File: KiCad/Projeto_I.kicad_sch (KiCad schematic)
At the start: 43 parts, among them J1 PORTA, J2 PORTB, J3 PORTC, J4 USB, J5 Barrel_Jack_Switch, Q1 PMOS, SW1 reset, U1 PIC18F4550-IP, U2 LM7805, U3 LM358, U4 AMS1117, U5 USBLC6-2SC6, Y1 16MHz

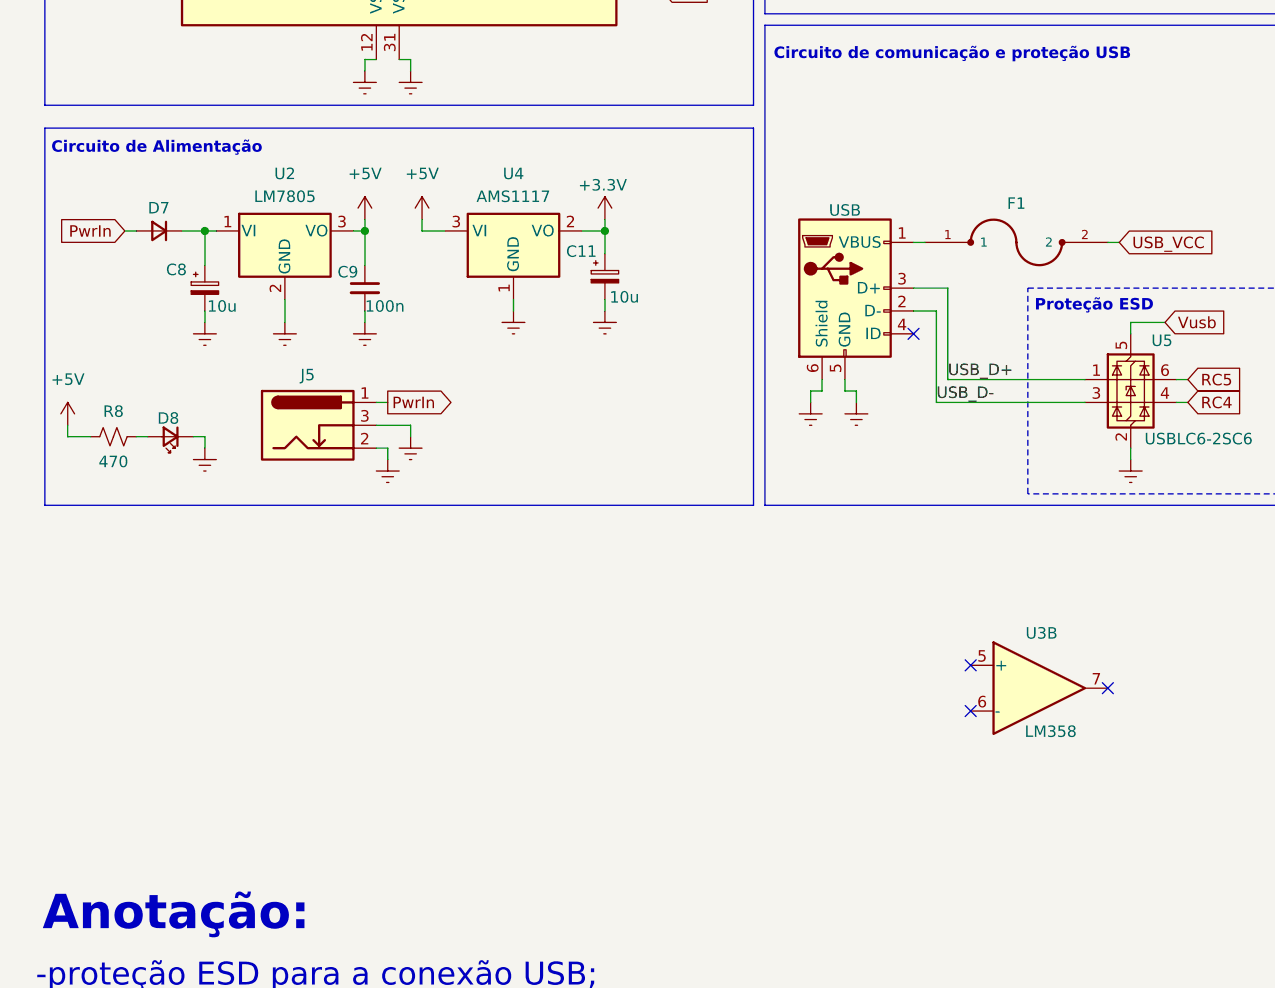
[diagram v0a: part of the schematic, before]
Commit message: Atualização da PCB
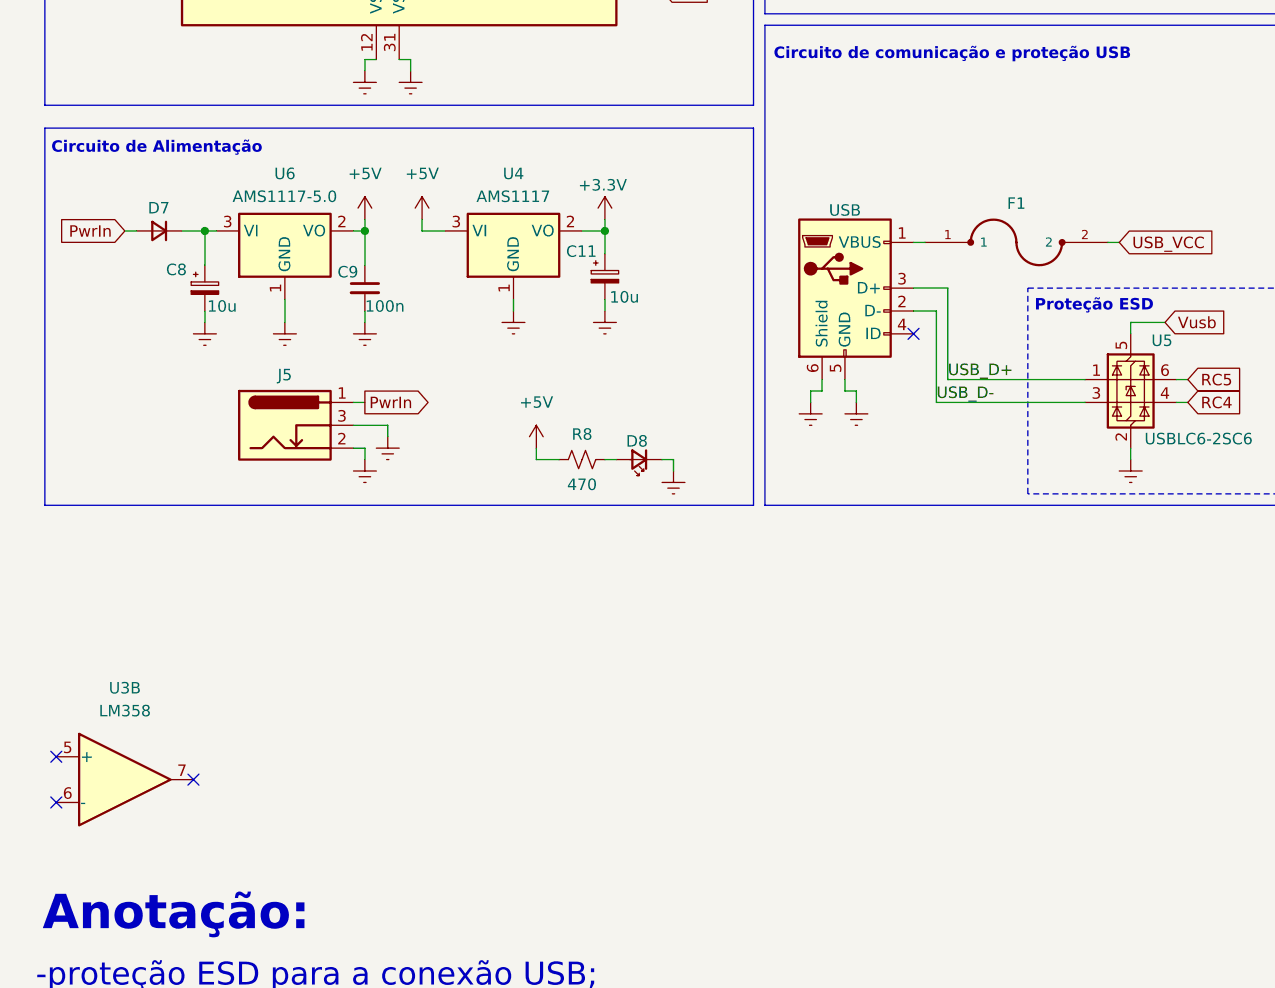
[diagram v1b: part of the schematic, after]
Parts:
- removed U2: LM7805, Package_TO_SOT_THT:TO-220-3_Vertical, symbol Regulator_Linear:LM7805_TO220
- added U6: AMS1117-5.0, Package_TO_SOT_SMD:SOT-223-3_TabPin2, symbol Regulator_Linear:AMS1117-5.0
- C1, C2: footprint Capacitor_THT:C_Rect_L7.0mm_W2.5mm_P5.00mm -> Capacitor_THT:C_Disc_D5.0mm_W2.5mm_P2.50mm
- C11, C8: footprint Capacitor_THT:CP_Radial_D10.0mm_P3.80mm -> Capacitor_THT:CP_Radial_D5.0mm_P2.50mm
- Q1: footprint Package_TO_SOT_THT:TO-92L_HandSolder -> Package_TO_SOT_SMD:SOT-23
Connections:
- net +5V: now also U6.2 (VO)
- net Earth: now also U6.1 (GND)
- net at C8.1, D7.1 (K): now also U6.3 (VI)
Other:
- moved on the sheet: D8, J5, R8
